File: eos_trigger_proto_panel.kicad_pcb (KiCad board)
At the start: 2 copper layers, 70.8 x 38.2 mm, 67 parts, among them J1 Conn_01x02, J2 Conn_01x02, J3 Conn_01x03, J4 Conn_01x02, U2 AD8099, U3 LTC6752-1, U4 SMA-Mylibrary, U5 SMA-Mylibrary

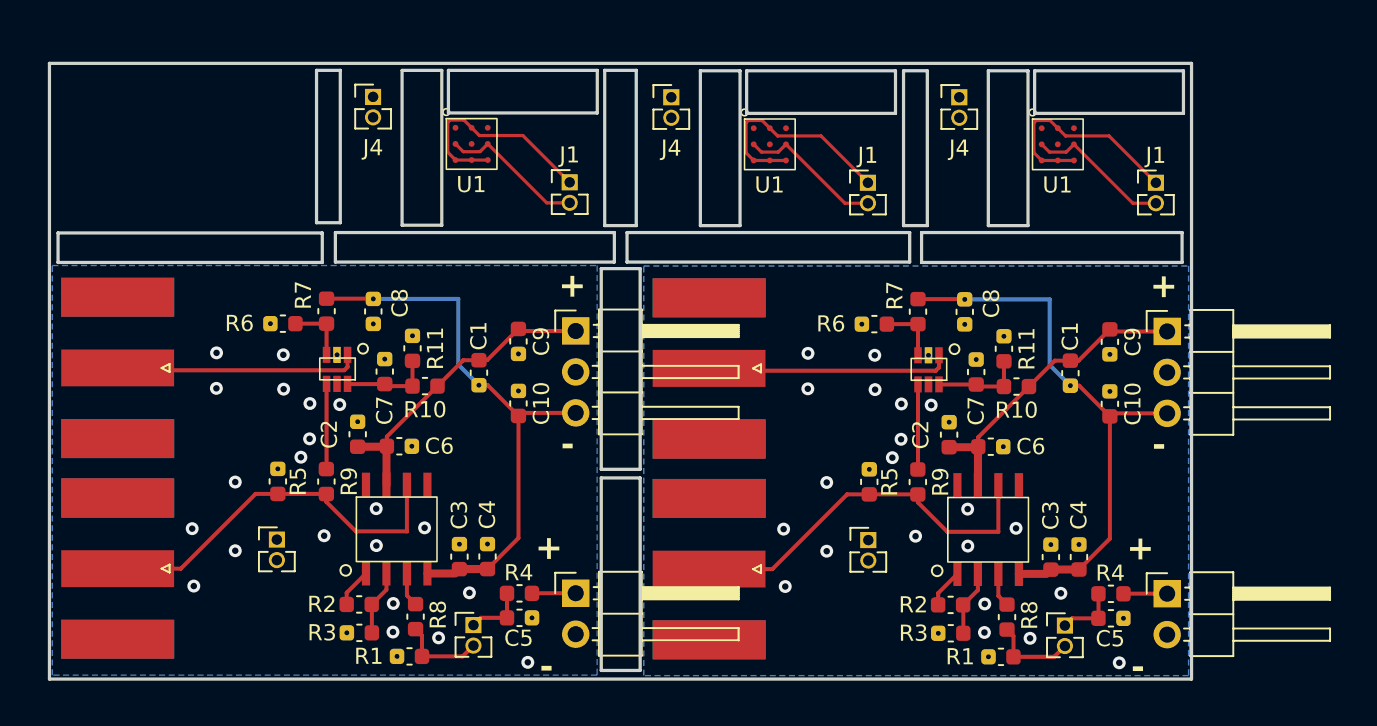
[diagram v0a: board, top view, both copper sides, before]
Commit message: update panel
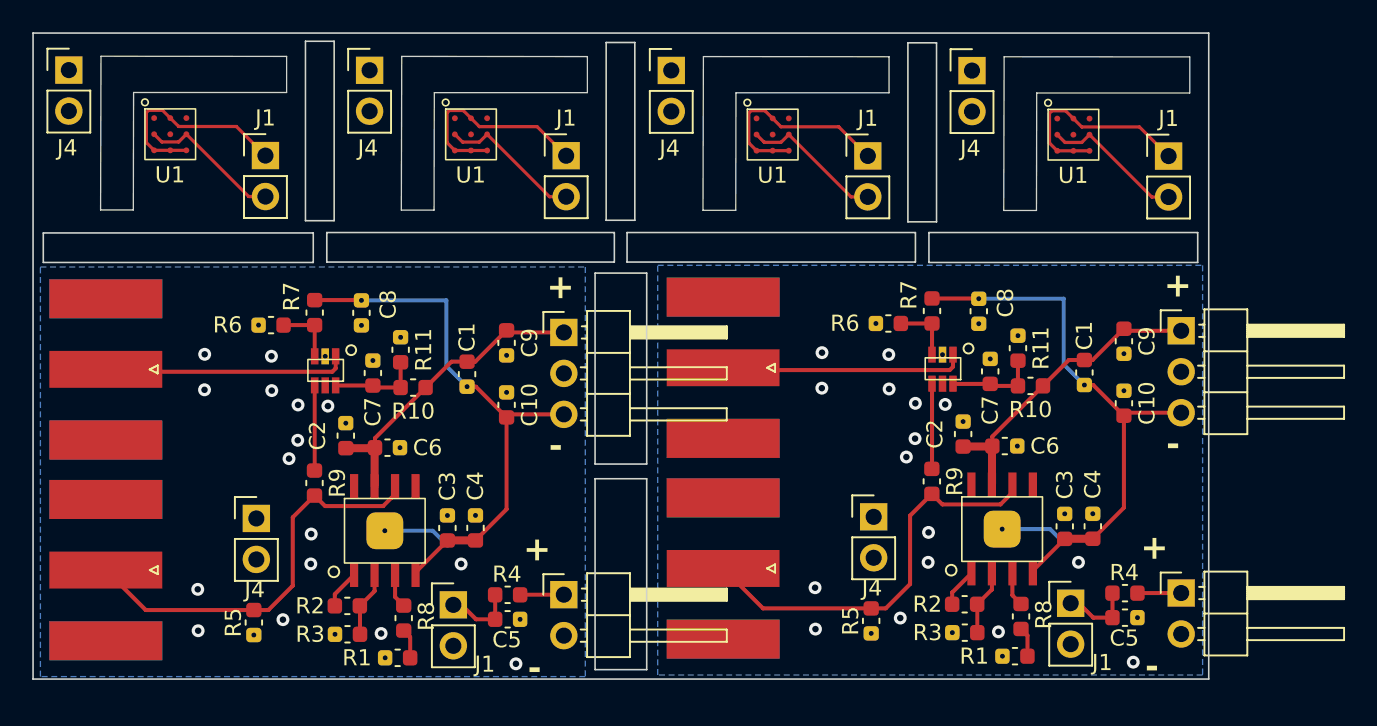
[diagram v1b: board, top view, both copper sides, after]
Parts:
- removed the C1 at (165.5, 89.0)
- removed the C1 at (202.2, 89.0)
- removed the C10 at (168.0, 90.9)
- removed the C10 at (204.7, 90.9)
- removed the C2 at (194.7, 92.8)
- removed the C2 at (158.0, 92.8)
- removed the C3 at (164.3, 100.4)
- removed the C3 at (201.0, 100.4)
- removed the C4 at (166.1, 100.4)
- removed the C4 at (202.7, 100.4)
- removed the C5 at (168.1, 104.2)
- removed the C5 at (204.7, 104.2)
- removed the C6 at (197.3, 93.5)
- removed the C6 at (160.6, 93.5)
- removed the C7 at (196.4, 88.9)
- removed the C7 at (159.7, 88.9)
- removed the C8 at (195.7, 85.2)
- removed the C8 at (159.0, 85.2)
- removed the C9 at (168.0, 87.0)
- removed the C9 at (204.7, 87.0)
- removed the J1 at (207.5, 77.2)
- removed the J1 at (189.7, 77.2)
- removed the J1 at (201.9, 104.6)
- removed the J1 at (165.2, 104.6)
- removed the J1 at (171.2, 77.2)
- removed the J2 at (208.2, 102.7)
- removed the J2 at (171.5, 102.6)
- removed the J3 at (208.2, 86.4)
- removed the J3 at (171.5, 86.4)
- removed the J4 at (153.0, 99.3)
- removed the J4 at (177.5, 71.9)
- removed the J4 at (159.0, 71.9)
- removed the J4 at (195.3, 71.9)
- removed the J4 at (189.7, 99.3)
- removed the R1 at (197.9, 106.6)
- removed the R1 at (161.2, 106.5)
- removed the R10 at (198.9, 89.8)
- removed the R10 at (162.2, 89.8)
- removed the R11 at (161.4, 87.4)
- removed the R11 at (198.1, 87.5)
- removed the R2 at (194.8, 103.4)
- removed the R2 at (158.1, 103.3)
- removed the R3 at (194.8, 105.1)
- removed the R3 at (158.1, 105.1)
- removed the R4 at (168.1, 102.6)
- removed the R4 at (204.7, 102.7)
- removed the R5 at (153.1, 95.7)
- removed the R5 at (189.7, 95.7)
- removed the R6 at (190.1, 85.9)
- removed the R6 at (153.4, 85.9)
- removed the R7 at (192.8, 85.2)
- removed the R7 at (156.1, 85.1)
- removed the R8 at (161.6, 104.1)
- removed the R8 at (198.3, 104.1)
- removed the R9 at (156.1, 95.7)
- removed the R9 at (192.8, 95.7)
- removed the U1 at (199.9, 73.2)
- removed the U1 at (182.0, 73.2)
- removed the U1 at (163.5, 73.2)
- removed the U2 at (194.6, 96.7)
- removed the U2 at (157.9, 96.7)
- removed the U3 at (194.5, 89.4)
- removed the U3 at (157.9, 89.4)
- removed the U4 at (180.5, 101.1)
- removed the U4 at (143.9, 101.1)
- removed the U5 at (143.9, 88.7)
- removed the U5 at (180.5, 88.7)
- added C1: 0.1u, EOS_library:C_0603_1608Metric, F.Cu at (203.1, 88.9)
- added C1: 0.1u, EOS_library:C_0603_1608Metric, F.Cu at (164.8, 89.0)
- added C10: 4.7u, EOS_library:C_0603_1608Metric, F.Cu at (167.3, 90.9)
- added C10: 4.7u, EOS_library:C_0603_1608Metric, F.Cu at (205.5, 90.8)
- added C2: 10u, EOS_library:C_0603_1608Metric, F.Cu at (157.3, 92.9)
- added C2: 10u, EOS_library:C_0603_1608Metric, F.Cu at (195.6, 92.8)
- added C3: 10u, EOS_library:C_0603_1608Metric, F.Cu at (201.9, 98.5)
- added C3: 10u, EOS_library:C_0603_1608Metric, F.Cu at (163.6, 98.6)
- added C4: 0.1u, EOS_library:C_0603_1608Metric, F.Cu at (165.3, 98.6)
- added C4: 0.1u, EOS_library:C_0603_1608Metric, F.Cu at (203.6, 98.5)
- added C5: C, EOS_library:C_0603_1608Metric, F.Cu at (167.3, 104.2)
- added C5: C, EOS_library:C_0603_1608Metric, F.Cu at (205.6, 104.1)
- added C6: 0.1u, EOS_library:C_0603_1608Metric, F.Cu at (159.9, 93.6)
- added C6: 0.1u, EOS_library:C_0603_1608Metric, F.Cu at (198.2, 93.5)
- added C7: 10u, EOS_library:C_0603_1608Metric, F.Cu at (159.0, 89.0)
- added C7: 10u, EOS_library:C_0603_1608Metric, F.Cu at (197.2, 88.9)
- added C8: C, EOS_library:C_0603_1608Metric, F.Cu at (196.5, 85.1)
- added C8: C, EOS_library:C_0603_1608Metric, F.Cu at (158.3, 85.2)
- added C9: 4.7u, EOS_library:C_0603_1608Metric, F.Cu at (167.3, 87.1)
- added C9: 4.7u, EOS_library:C_0603_1608Metric, F.Cu at (205.5, 87.0)
- added J1: Conn_01x02, Connector_PinHeader_2.54mm:PinHeader_1x02_P2.54mm_Vertical, F.Cu at (202.2, 103.2)
- added J1: Conn_01x02, Connector_PinHeader_2.54mm:PinHeader_1x02_P2.54mm_Vertical, F.Cu at (152.3, 75.5)
- added J1: Conn_01x02, Connector_PinHeader_2.54mm:PinHeader_1x02_P2.54mm_Vertical, F.Cu at (208.3, 75.5)
- added J1: Conn_01x02, Connector_PinHeader_2.54mm:PinHeader_1x02_P2.54mm_Vertical, F.Cu at (171.0, 75.5)
- added J1: Conn_01x02, Connector_PinHeader_2.54mm:PinHeader_1x02_P2.54mm_Vertical, F.Cu at (164.0, 103.3)
- added J1: Conn_01x02, Connector_PinHeader_2.54mm:PinHeader_1x02_P2.54mm_Vertical, F.Cu at (189.7, 75.5)
- added J2: Conn_01x02, Connector_PinHeader_2.54mm:PinHeader_1x02_P2.54mm_Horizontal, F.Cu at (170.8, 102.7)
- added J2: Conn_01x02, Connector_PinHeader_2.54mm:PinHeader_1x02_P2.54mm_Horizontal, F.Cu at (209.1, 102.6)
- added J3: Conn_01x03, Connector_PinHeader_2.54mm:PinHeader_1x03_P2.54mm_Horizontal, F.Cu at (170.8, 86.5)
- added J3: Conn_01x03, Connector_PinHeader_2.54mm:PinHeader_1x03_P2.54mm_Horizontal, F.Cu at (209.1, 86.4)
- added J4: Conn_01x02, Connector_PinHeader_2.54mm:PinHeader_1x02_P2.54mm_Vertical, F.Cu at (158.8, 70.2)
- added J4: Conn_01x02, Connector_PinHeader_2.54mm:PinHeader_1x02_P2.54mm_Vertical, F.Cu at (140.1, 70.2)
- added J4: Conn_01x02, Connector_PinHeader_2.54mm:PinHeader_1x02_P2.54mm_Vertical, F.Cu at (196.1, 70.2)
- added J4: Conn_01x02, Connector_PinHeader_2.54mm:PinHeader_1x02_P2.54mm_Vertical, F.Cu at (151.7, 98.0)
- added J4: Conn_01x02, Connector_PinHeader_2.54mm:PinHeader_1x02_P2.54mm_Vertical, F.Cu at (177.5, 70.2)
- added J4: Conn_01x02, Connector_PinHeader_2.54mm:PinHeader_1x02_P2.54mm_Vertical, F.Cu at (190.0, 97.9)
- added R1: 49.9, EOS_library:C_0603_1608Metric, F.Cu at (198.8, 106.5)
- added R1: 49.9, EOS_library:C_0603_1608Metric, F.Cu at (160.5, 106.6)
- added R10: R, EOS_library:C_0603_1608Metric, F.Cu at (161.5, 89.9)
- added R10: R, EOS_library:C_0603_1608Metric, F.Cu at (199.7, 89.8)
- added R11: R, EOS_library:C_0603_1608Metric, F.Cu at (199.0, 87.4)
- added R11: R, EOS_library:C_0603_1608Metric, F.Cu at (160.7, 87.5)
- added R2: 499, EOS_library:C_0603_1608Metric, F.Cu at (195.7, 103.3)
- added R2: 499, EOS_library:C_0603_1608Metric, F.Cu at (157.4, 103.4)
- added R3: 13, EOS_library:C_0603_1608Metric, F.Cu at (195.7, 105.1)
- added R3: 13, EOS_library:C_0603_1608Metric, F.Cu at (157.4, 105.2)
- added R4: R, EOS_library:C_0603_1608Metric, F.Cu at (167.3, 102.7)
- added R4: R, EOS_library:C_0603_1608Metric, F.Cu at (205.6, 102.6)
- added R5: 49.9, EOS_library:C_0603_1608Metric, F.Cu at (151.6, 104.4)
- added R5: 49.9, EOS_library:C_0603_1608Metric, F.Cu at (189.9, 104.3)
- added R6: R, EOS_library:C_0603_1608Metric, F.Cu at (190.9, 85.9)
- added R6: R, EOS_library:C_0603_1608Metric, F.Cu at (152.7, 86.0)
- added R7: R, EOS_library:C_0603_1608Metric, F.Cu at (155.4, 85.2)
- added R7: R, EOS_library:C_0603_1608Metric, F.Cu at (193.6, 85.1)
- added R8: 0, EOS_library:C_0603_1608Metric, F.Cu at (199.2, 104.1)
- added R8: 0, EOS_library:C_0603_1608Metric, F.Cu at (160.9, 104.2)
- added R9: 0, EOS_library:C_0603_1608Metric, F.Cu at (155.3, 95.8)
- added R9: 0, EOS_library:C_0603_1608Metric, F.Cu at (193.6, 95.7)
- added U1: ~, EOS_library:AFBR-S4N33C013, F.Cu at (182.2, 72.6)
- added U1: ~, EOS_library:AFBR-S4N33C013, F.Cu at (163.5, 72.6)
- added U1: ~, EOS_library:AFBR-S4N33C013, F.Cu at (144.8, 72.6)
- added U1: ~, EOS_library:AFBR-S4N33C013, F.Cu at (200.8, 72.6)
- added U2: AD8099, EOS_library:AD8099, F.Cu at (157.2, 96.8)
- added U2: AD8099, EOS_library:AD8099, F.Cu at (195.5, 96.7)
- added U3: LTC6752-1, EOS_library:LT6752-1, F.Cu at (195.4, 89.4)
- added U3: LTC6752-1, EOS_library:LT6752-1, F.Cu at (157.1, 89.5)
- added U4: SMA-Mylibrary, EOS_library:SMA_Molex_73251-1153_EdgeMount_Horizontal, F.Cu at (143.1, 101.2)
- added U4: SMA-Mylibrary, EOS_library:SMA_Molex_73251-1153_EdgeMount_Horizontal, F.Cu at (181.4, 101.1)
- added U5: SMA-Mylibrary, EOS_library:SMA_Molex_73251-1153_EdgeMount_Horizontal, F.Cu at (181.4, 88.6)
- added U5: SMA-Mylibrary, EOS_library:SMA_Molex_73251-1153_EdgeMount_Horizontal, F.Cu at (143.1, 88.7)
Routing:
- net /IN: track 41.3 -> 52.6 mm
- net SIG OUT: track 48.0 -> 57.2 mm
- net /OUT: track 27.0 -> 35.6 mm
- net GND: track 0.00 -> 8.54 mm, vias 42 -> 32
- net /SiPM_daughter/OUT: track 10.6 -> 3.71 mm
- net -5V: track 69.3 -> 68.1 mm
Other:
- board size 70.8 x 38.2 mm -> 72.9 x 40.1 mm

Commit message: tweaks
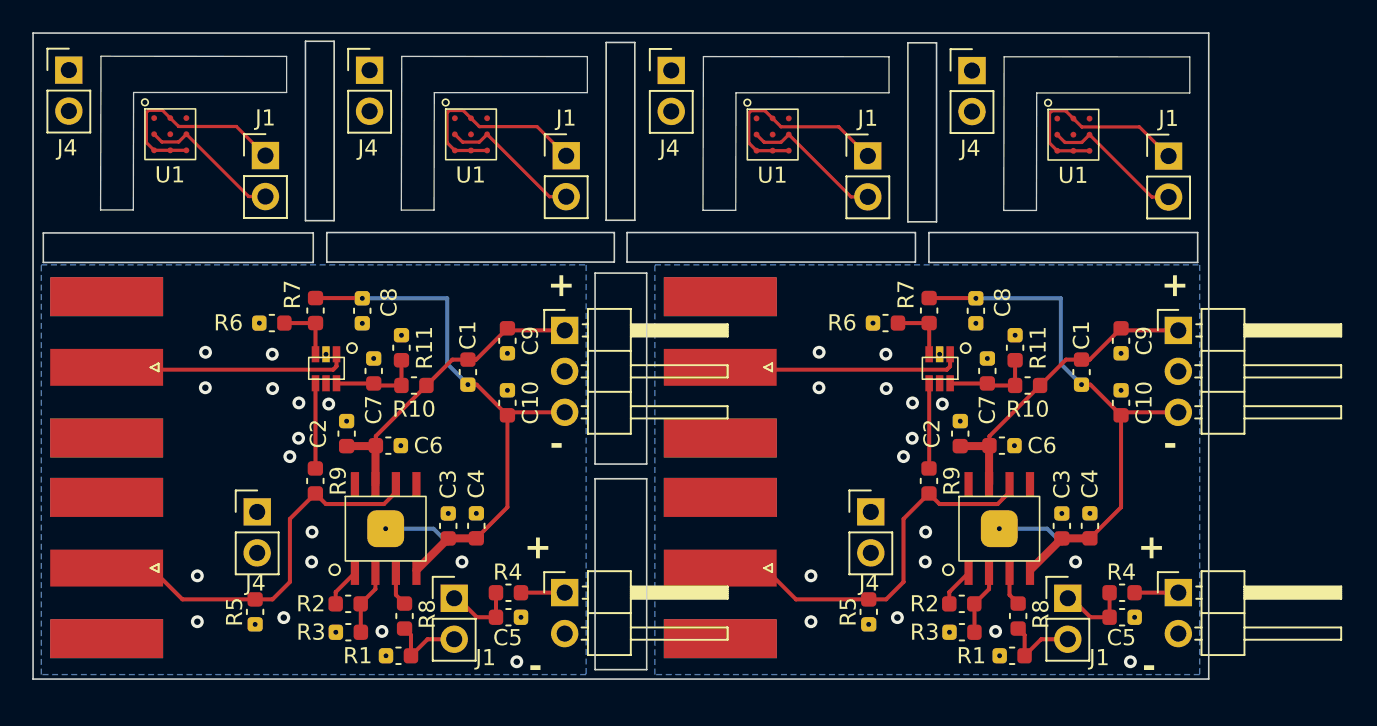
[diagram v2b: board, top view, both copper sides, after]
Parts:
- removed the C1 at (203.1, 88.9)
- removed the C1 at (164.8, 89.0)
- removed the C10 at (167.3, 90.9)
- removed the C10 at (205.5, 90.8)
- removed the C2 at (157.3, 92.9)
- removed the C2 at (195.6, 92.8)
- removed the C3 at (201.9, 98.5)
- removed the C3 at (163.6, 98.6)
- removed the C4 at (165.3, 98.6)
- removed the C4 at (203.6, 98.5)
- removed the C5 at (167.3, 104.2)
- removed the C5 at (205.6, 104.1)
- removed the C6 at (159.9, 93.6)
- removed the C6 at (198.2, 93.5)
- removed the C7 at (159.0, 89.0)
- removed the C7 at (197.2, 88.9)
- removed the C8 at (196.5, 85.1)
- removed the C8 at (158.3, 85.2)
- removed the C9 at (167.3, 87.1)
- removed the C9 at (205.5, 87.0)
- removed the J1 at (202.2, 103.2)
- removed the J1 at (164.0, 103.3)
- removed the J2 at (170.8, 102.7)
- removed the J2 at (209.1, 102.6)
- removed the J3 at (170.8, 86.5)
- removed the J3 at (209.1, 86.4)
- removed the J4 at (151.7, 98.0)
- removed the J4 at (190.0, 97.9)
- removed the R1 at (198.8, 106.5)
- removed the R1 at (160.5, 106.6)
- removed the R10 at (161.5, 89.9)
- removed the R10 at (199.7, 89.8)
- removed the R11 at (199.0, 87.4)
- removed the R11 at (160.7, 87.5)
- removed the R2 at (195.7, 103.3)
- removed the R2 at (157.4, 103.4)
- removed the R3 at (195.7, 105.1)
- removed the R3 at (157.4, 105.2)
- removed the R4 at (167.3, 102.7)
- removed the R4 at (205.6, 102.6)
- removed the R5 at (151.6, 104.4)
- removed the R5 at (189.9, 104.3)
- removed the R6 at (190.9, 85.9)
- removed the R6 at (152.7, 86.0)
- removed the R7 at (155.4, 85.2)
- removed the R7 at (193.6, 85.1)
- removed the R8 at (199.2, 104.1)
- removed the R8 at (160.9, 104.2)
- removed the R9 at (155.3, 95.8)
- removed the R9 at (193.6, 95.7)
- removed the U2 at (157.2, 96.8)
- removed the U2 at (195.5, 96.7)
- removed the U3 at (195.4, 89.4)
- removed the U3 at (157.1, 89.5)
- removed the U4 at (143.1, 101.2)
- removed the U4 at (181.4, 101.1)
- removed the U5 at (181.4, 88.6)
- removed the U5 at (143.1, 88.7)
- added C1: 0.1u, EOS_library:C_0603_1608Metric, F.Cu at (202.9, 88.9)
- added C1: 0.1u, EOS_library:C_0603_1608Metric, F.Cu at (164.9, 88.9)
- added C10: 4.7u, EOS_library:C_0603_1608Metric, F.Cu at (205.4, 90.8)
- added C10: 4.7u, EOS_library:C_0603_1608Metric, F.Cu at (167.3, 90.8)
- added C2: 10u, EOS_library:C_0603_1608Metric, F.Cu at (157.3, 92.7)
- added C2: 10u, EOS_library:C_0603_1608Metric, F.Cu at (195.4, 92.7)
- added C3: 10u, EOS_library:C_0603_1608Metric, F.Cu at (201.7, 98.5)
- added C3: 10u, EOS_library:C_0603_1608Metric, F.Cu at (163.6, 98.5)
- added C4: 0.1u, EOS_library:C_0603_1608Metric, F.Cu at (165.4, 98.5)
- added C4: 0.1u, EOS_library:C_0603_1608Metric, F.Cu at (203.4, 98.5)
- added C5: C, EOS_library:C_0603_1608Metric, F.Cu at (167.4, 104.1)
- added C5: C, EOS_library:C_0603_1608Metric, F.Cu at (205.4, 104.1)
- added C6: 0.1u, EOS_library:C_0603_1608Metric, F.Cu at (198.0, 93.5)
- added C6: 0.1u, EOS_library:C_0603_1608Metric, F.Cu at (159.9, 93.5)
- added C7: 10u, EOS_library:C_0603_1608Metric, F.Cu at (197.1, 88.8)
- added C7: 10u, EOS_library:C_0603_1608Metric, F.Cu at (159.0, 88.8)
- added C8: C, EOS_library:C_0603_1608Metric, F.Cu at (196.4, 85.1)
- added C8: C, EOS_library:C_0603_1608Metric, F.Cu at (158.3, 85.1)
- added C9: 4.7u, EOS_library:C_0603_1608Metric, F.Cu at (167.3, 87.0)
- added C9: 4.7u, EOS_library:C_0603_1608Metric, F.Cu at (205.4, 87.0)
- added J1: Conn_01x02, Connector_PinHeader_2.54mm:PinHeader_1x02_P2.54mm_Vertical, F.Cu at (164.0, 102.9)
- added J1: Conn_01x02, Connector_PinHeader_2.54mm:PinHeader_1x02_P2.54mm_Vertical, F.Cu at (202.1, 102.9)
- added J2: Conn_01x02, Connector_PinHeader_2.54mm:PinHeader_1x02_P2.54mm_Horizontal, F.Cu at (208.9, 102.6)
- added J2: Conn_01x02, Connector_PinHeader_2.54mm:PinHeader_1x02_P2.54mm_Horizontal, F.Cu at (170.9, 102.6)
- added J3: Conn_01x03, Connector_PinHeader_2.54mm:PinHeader_1x03_P2.54mm_Horizontal, F.Cu at (170.9, 86.3)
- added J3: Conn_01x03, Connector_PinHeader_2.54mm:PinHeader_1x03_P2.54mm_Horizontal, F.Cu at (208.9, 86.3)
- added J4: Conn_01x02, Connector_PinHeader_2.54mm:PinHeader_1x02_P2.54mm_Vertical, F.Cu at (151.8, 97.6)
- added J4: Conn_01x02, Connector_PinHeader_2.54mm:PinHeader_1x02_P2.54mm_Vertical, F.Cu at (189.8, 97.6)
- added R1: 49.9, EOS_library:C_0603_1608Metric, F.Cu at (160.6, 106.5)
- added R1: 49.9, EOS_library:C_0603_1608Metric, F.Cu at (198.6, 106.5)
- added R10: R, EOS_library:C_0603_1608Metric, F.Cu at (199.6, 89.7)
- added R10: R, EOS_library:C_0603_1608Metric, F.Cu at (161.5, 89.7)
- added R11: R, EOS_library:C_0603_1608Metric, F.Cu at (160.7, 87.4)
- added R11: R, EOS_library:C_0603_1608Metric, F.Cu at (198.8, 87.4)
- added R2: 499, EOS_library:C_0603_1608Metric, F.Cu at (195.5, 103.3)
- added R2: 499, EOS_library:C_0603_1608Metric, F.Cu at (157.4, 103.3)
- added R3: 13, EOS_library:C_0603_1608Metric, F.Cu at (157.4, 105.0)
- added R3: 13, EOS_library:C_0603_1608Metric, F.Cu at (195.5, 105.0)
- added R4: R, EOS_library:C_0603_1608Metric, F.Cu at (205.4, 102.6)
- added R4: R, EOS_library:C_0603_1608Metric, F.Cu at (167.4, 102.6)
- added R5: 49.9, EOS_library:C_0603_1608Metric, F.Cu at (151.7, 103.8)
- added R5: 49.9, EOS_library:C_0603_1608Metric, F.Cu at (189.7, 103.8)
- added R6: R, EOS_library:C_0603_1608Metric, F.Cu at (190.8, 85.9)
- added R6: R, EOS_library:C_0603_1608Metric, F.Cu at (152.7, 85.9)
- added R7: R, EOS_library:C_0603_1608Metric, F.Cu at (155.4, 85.1)
- added R7: R, EOS_library:C_0603_1608Metric, F.Cu at (193.5, 85.1)
- added R8: 0, EOS_library:C_0603_1608Metric, F.Cu at (160.9, 104.0)
- added R8: 0, EOS_library:C_0603_1608Metric, F.Cu at (199.0, 104.0)
- added R9: 0, EOS_library:C_0603_1608Metric, F.Cu at (193.4, 95.7)
- added R9: 0, EOS_library:C_0603_1608Metric, F.Cu at (155.4, 95.7)
- added U2: AD8099, EOS_library:AD8099, F.Cu at (157.3, 96.6)
- added U2: AD8099, EOS_library:AD8099, F.Cu at (195.3, 96.6)
- added U3: LTC6752-1, EOS_library:LT6752-1, F.Cu at (195.2, 89.4)
- added U3: LTC6752-1, EOS_library:LT6752-1, F.Cu at (157.2, 89.4)
- added U4: SMA-Mylibrary, EOS_library:SMA_Molex_73251-1153_EdgeMount_Horizontal, F.Cu at (143.2, 101.1)
- added U4: SMA-Mylibrary, EOS_library:SMA_Molex_73251-1153_EdgeMount_Horizontal, F.Cu at (181.2, 101.1)
- added U5: SMA-Mylibrary, EOS_library:SMA_Molex_73251-1153_EdgeMount_Horizontal, F.Cu at (143.2, 88.6)
- added U5: SMA-Mylibrary, EOS_library:SMA_Molex_73251-1153_EdgeMount_Horizontal, F.Cu at (181.2, 88.6)
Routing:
- net /SiPM_daughter/OUT: track 3.71 -> 9.92 mm
- net SIG OUT: track 57.2 -> 56.0 mm
